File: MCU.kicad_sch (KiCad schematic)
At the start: 21 parts

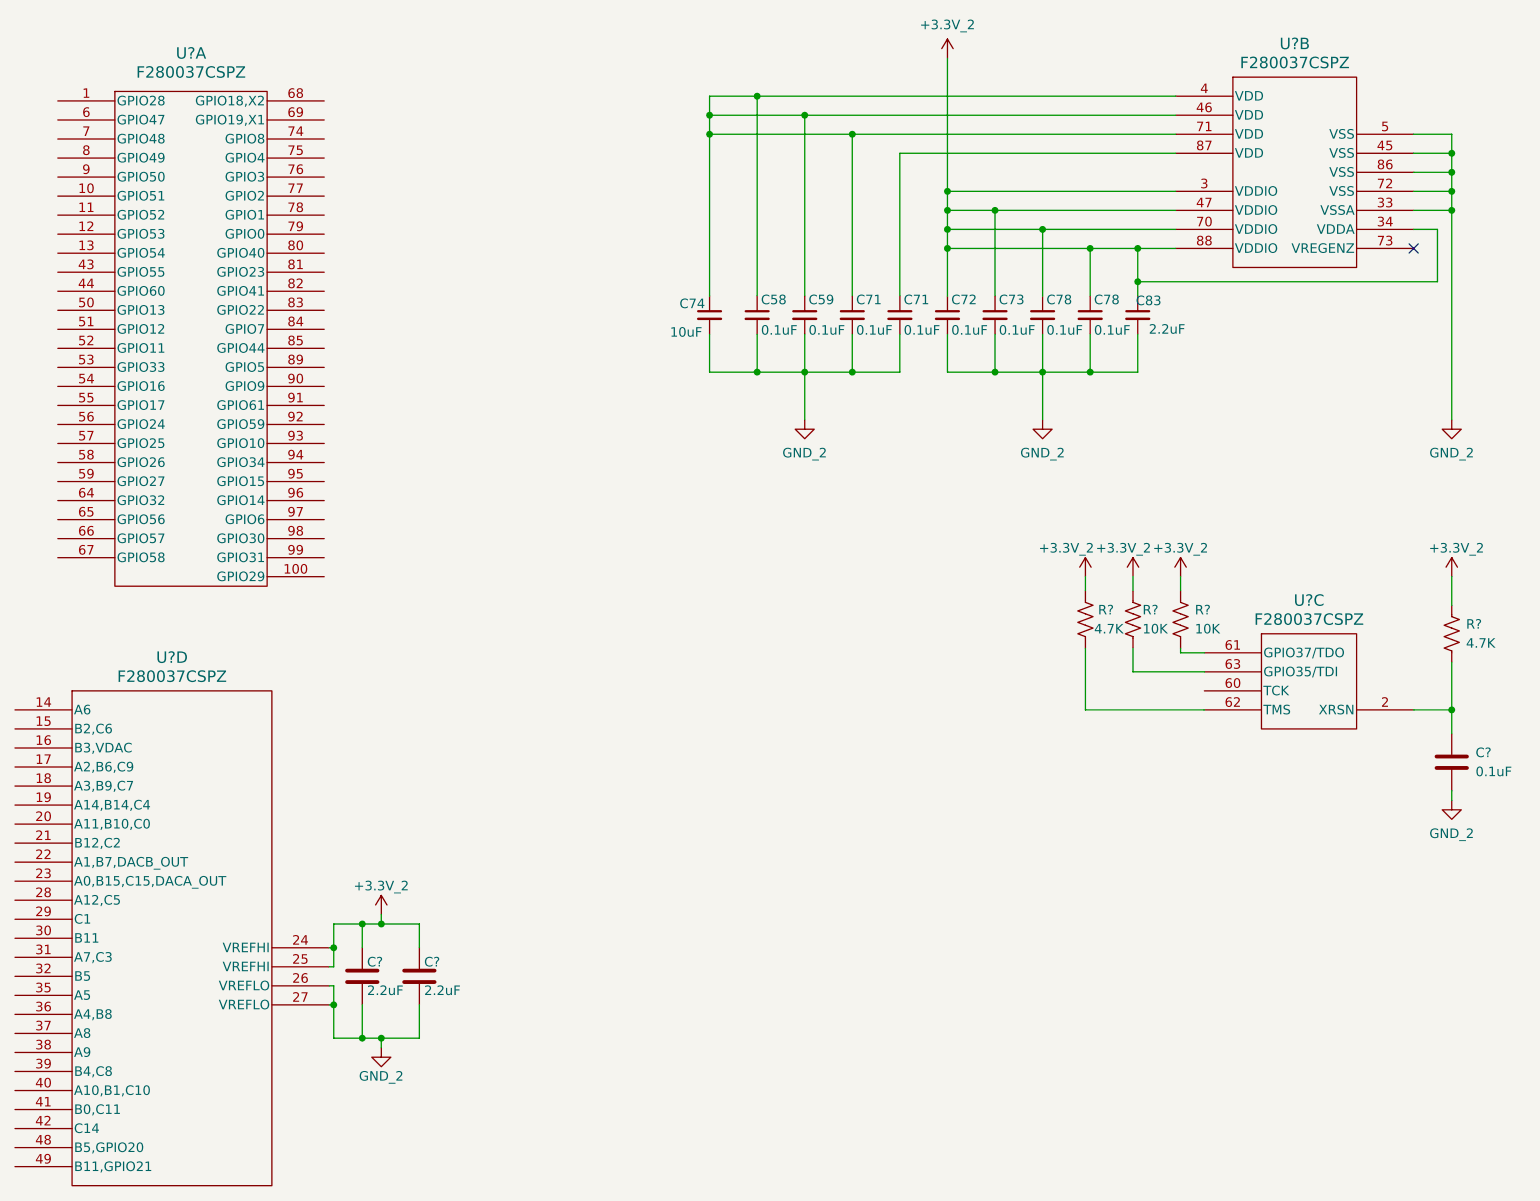
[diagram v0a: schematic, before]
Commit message: MCU updated to 48 pin
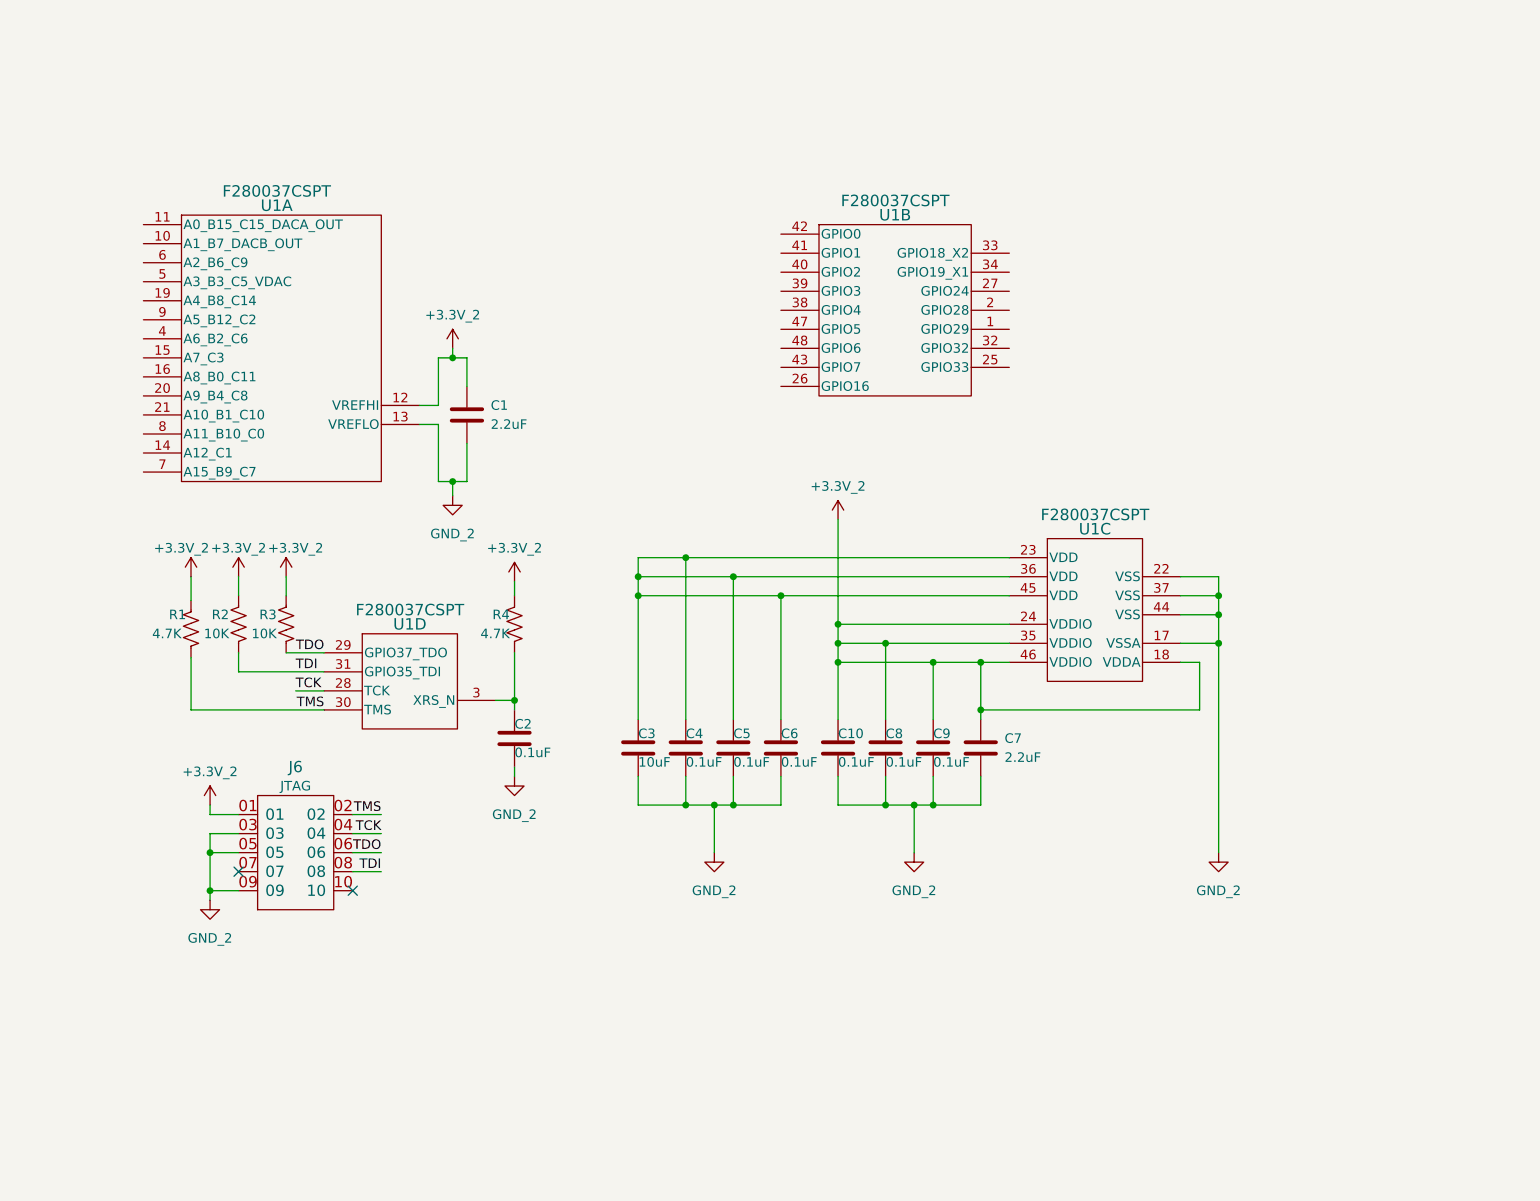
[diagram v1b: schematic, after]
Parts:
- removed C58, C59, C71 (x2), C72, C73, C78 (x2): 0.1uF, Power_Analyzer:C_0603_1608Metric, symbol Power_Analyzer:0.1uF
- removed C74: 10uF, Power_Analyzer:C_0805_2012Metric, symbol Power_Analyzer:10uF
- removed C83: 2.2uF, Power_Analyzer:C_0603_1608Metric, symbol Power_Analyzer:2.2uF
- removed C?: 0.1uF, Capacitor_SMD:C_0603_1608Metric, symbol Major_Project:0.1uF
- removed C? (x2): 2.2uF, Capacitor_SMD:C_0603_1608Metric, symbol Major_Project:2.2uF
- removed R? (x2): 4.7K, Resistor_SMD:R_1206_3216Metric, symbol Major_Project:4.7K
- removed R? (x2): 10K, Resistor_SMD:R_1206_3216Metric, symbol Major_Project:10K
- removed U? (x4): F280037CSPZ, LQFP100_PZ_TEX, symbol Major_Project:F280037CSPZ
- added C1, C7: 2.2uF, Capacitor_SMD:C_0603_1608Metric, symbol Major_Project:2.2uF
- added C10, C2, C4, C5, C6, C8, C9: 0.1uF, Capacitor_SMD:C_0603_1608Metric, symbol Major_Project:0.1uF
- added C3: 10uF, Capacitor_SMD:C_0603_1608Metric, symbol Major_Project:10uF
- added J6: JTAG, Power_Analyzer:SAMTEC_FTSH-105-01-F-DV-K, symbol Power_Analyzer:FTSH-105-01-F-DV-K
- added R1, R4: 4.7K, Resistor_SMD:R_1206_3216Metric, symbol Major_Project:4.7K
- added R2, R3: 10K, Resistor_SMD:R_1206_3216Metric, symbol Major_Project:10K
- added U1: F280037CSPT, Power_Analyzer:PT0048A-MFG, symbol Major_Project:F280037CSPT
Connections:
- net +3.3V_2: now also C1.1, C10.1, C7.1, C8.1, C9.1, J6.01, R1.1, R2.1, R3.1, R4.1, U1.12 (VREFHI), U1.18 (VDDA), U1.24 (VDDIO), U1.35 (VDDIO), U1.46 (VDDIO)
- net GND_2: now also C1.2, C10.2, C2.2, C3.2, C4.2, C5.2, C6.2, C7.2, C8.2, C9.2, J6.03, J6.05, J6.09, U1.13 (VREFLO), U1.17 (VSSA), U1.22 (VSS), U1.37 (VSS), U1.44 (VSS)
- new net: C3.1, C4.1, C5.1, C6.1, U1.23 (VDD), U1.36 (VDD), U1.45 (VDD)
- new net: C2.1, R4.2, U1.3 (XRS_N)
- new net TCK: J6.04, U1.28 (TCK)
- new net TDI: J6.08, R2.2, U1.31 (GPIO35_TDI)
- new net TDO: J6.06, R3.2, U1.29 (GPIO37_TDO)
- new net TMS: J6.02, R1.2, U1.30 (TMS)
- no-connect marks 1 -> 2
